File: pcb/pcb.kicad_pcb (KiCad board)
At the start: 2 copper layers, 41.2 x 25.6 mm, 32 parts, among them J1 Conn_01x02, J2 Conn_01x02, SW1 SW_SPDT, U1 TL072, U3 AP63205WU

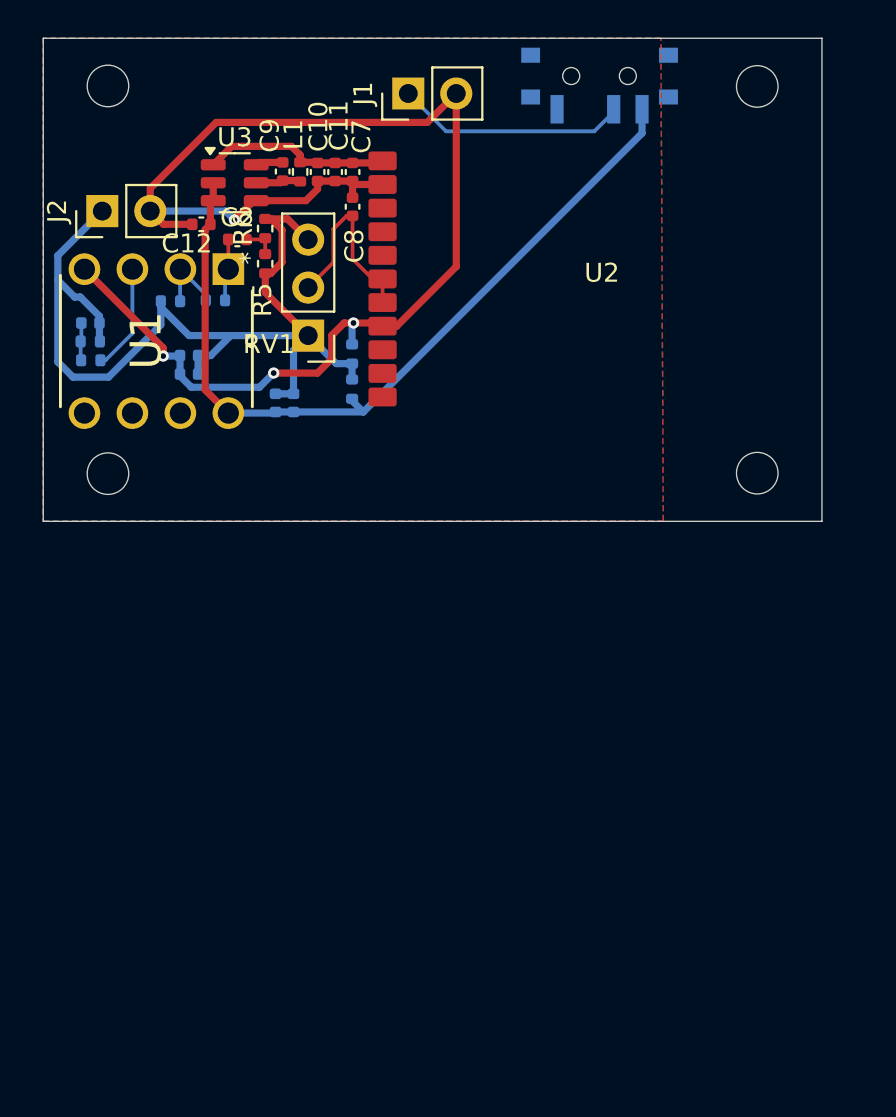
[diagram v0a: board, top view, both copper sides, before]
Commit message: pcb v2
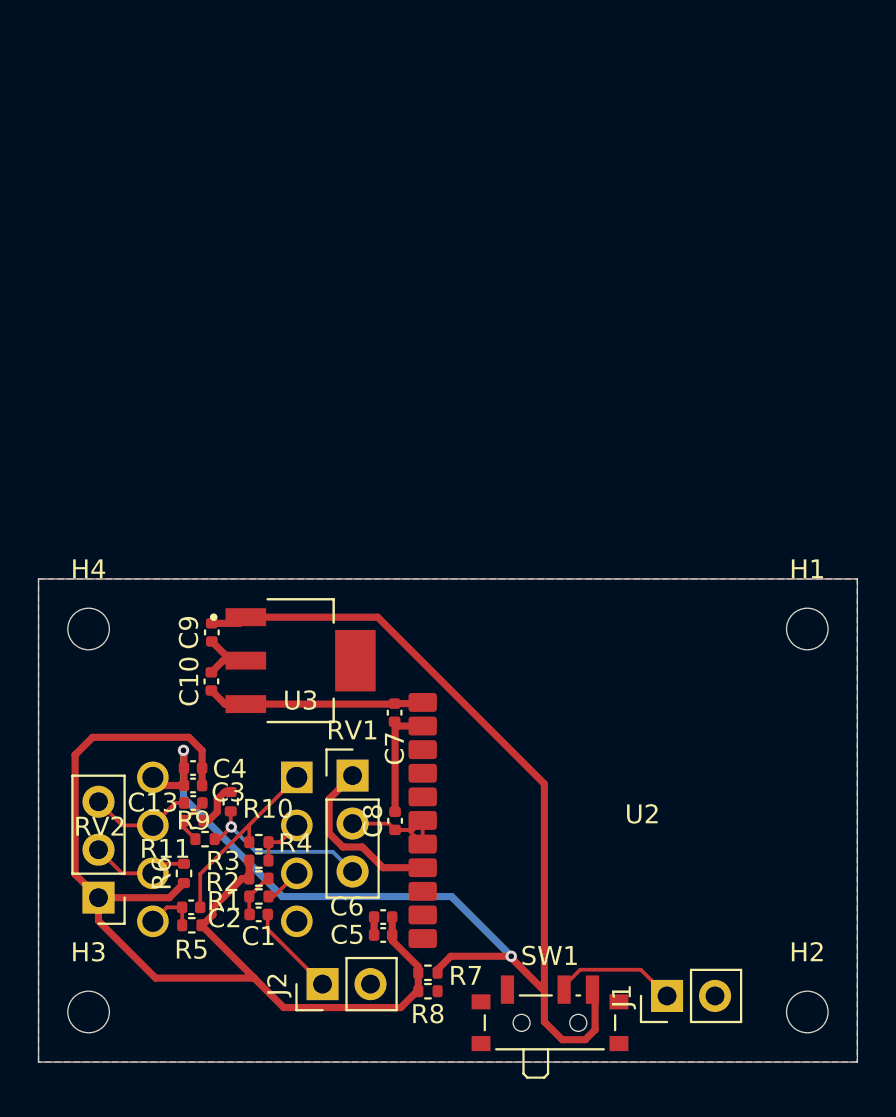
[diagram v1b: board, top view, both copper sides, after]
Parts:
- removed C11: 22u, Capacitor_SMD:C_0402_1005Metric
- removed C12: 10u, Capacitor_SMD:C_0402_1005Metric
- removed L1: 4u7, Resistor_SMD:R_0402_1005Metric
- added C13: 1u, Capacitor_SMD:C_0402_1005Metric, F.Cu at (90.7, 64.1)
- added R10: 4k7, Resistor_SMD:R_0402_1005Metric, F.Cu at (92.7, 64.0)
- added R11: 10k, Resistor_SMD:R_0402_1005Metric, F.Cu at (91.3, 66.0)
- added R9: 100k, Resistor_SMD:R_0402_1005Metric, F.Cu at (90.7, 65.0)
- added RV2: 100k, Connector_PinHeader_2.54mm:PinHeader_1x03_P2.54mm_Vertical, F.Cu at (85.7, 69.1)
- C1, C3, C4, C5, C6, R2, R4, R7, R8, SW1: moved to F.Cu
- C10: value 22u -> 0.1u
- C9: value 100n -> 0.22u
- R1: value 1M -> 1k; moved to F.Cu
- R3: value 10k -> 5k; moved to F.Cu
- R6: value 47 -> 10k
- RV1: value R_Potentiometer -> 100k
- U1: moved to B.Cu
- U3: value AP63205WU -> LM7805_TO220; footprint Package_TO_SOT_SMD:TSOT-23-6 -> LM7805MP_NOPB:VREG_LM7805MP_NOPB
- moved J1 49.7 mm to (115.8, 74.3)
- moved SW1 49.5 mm to (109.5, 75.4)
- moved H2 49.1 mm to (123.2, 75.1)
- moved H3 49.0 mm to (85.1, 75.1)
- moved J2 42.6 mm to (97.5, 73.7)
- moved C2 35.4 mm to (90.6, 69.6), turned to 180 degrees
- moved R5 35.2 mm to (90.6, 70.5), turned to 0 degrees
- moved R6 34.4 mm to (90.2, 67.8)
- moved R8 34.0 mm to (103.1, 74.0), turned to 0 degrees
- moved C8 32.6 mm to (101.3, 65.0)
- moved C1 32.6 mm to (94.1, 70.0)
- moved C5 32.4 mm to (100.7, 71.0)
- moved R7 31.2 mm to (103.1, 73.0), turned to 180 degrees
- moved C6 30.5 mm to (100.7, 70.1)
- moved R3 30.0 mm to (94.1, 67.1)
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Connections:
- C1 pad 1: GND -> Net-(J2-Pin_1)
- C2 pad 2: Net-(C2-Pad2) -> Net-(U1B-+)
- C9 pad 1: Net-(U3-SW) -> +9V
- C9 pad 2: Net-(U3-BST) -> GNDPWR
- J2 pad 1: GND -> Net-(J2-Pin_1)
- R5 pad 1: Net-(C2-Pad2) -> Net-(U1B-+)
- R6 pad 1: Net-(C2-Pad2) -> GND
- R6 pad 2: GND -> Net-(U1B--)
- RV1 pad 1: GND -> GNDPWR
- RV1 pad 3: GND -> Net-(R10-Pad1)
- U1 pad 5: unconnected-(U1B-+-Pad5) -> Net-(U1B-+)
- U1 pad 6: unconnected-(U1B---Pad6) -> Net-(U1B--)
- U1 pad 7: unconnected-(U1-Pad7) -> Net-(C13-Pad1)
- U3 pad 1: +5V -> +9V
- U3 pad 2: +9V -> GNDPWR
- U3 pad 3: +9V -> +5V
- U3 pad 4: GNDPWR -> (no net)
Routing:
- net GNDPWR: track 73.6 -> 23.4 mm, vias 4 -> 0
- net +9V: track 43.1 -> 73.4 mm, vias 0 -> 2
- net Net-(R10-Pad1): track 0.00 -> 9.39 mm, vias 0 -> 1
- net Net-(C2-Pad1): track 3.30 -> 9.91 mm
- net Net-(J1-Pin_1): track 12.3 -> 6.58 mm
- net Net-(C13-Pad1): track 0.00 -> 5.55 mm
- net Net-(U1B--): track 0.00 -> 5.25 mm
- net Net-(J2-Pin_1): track 0.00 -> 4.89 mm
- net Net-(U1A-+): track 5.69 -> 2.01 mm
- net Net-(U2-AUDIO_L): track 10.5 -> 7.08 mm
- net GND: track 52.4 -> 55.8 mm
- net Net-(U1B-+): track 0.00 -> 2.80 mm
- net Net-(C13-Pad2): track 0.00 -> 2.58 mm
- net Net-(U3-SW): track 2.39 -> 0.00 mm
- net Net-(C2-Pad2): track 1.86 -> 0.00 mm
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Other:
- board size 41.2 x 25.6 mm -> 43.4 x 25.6 mm
